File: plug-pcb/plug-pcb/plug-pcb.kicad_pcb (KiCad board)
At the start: 2 copper layers, 1 part, among them J2 Conn_01x05

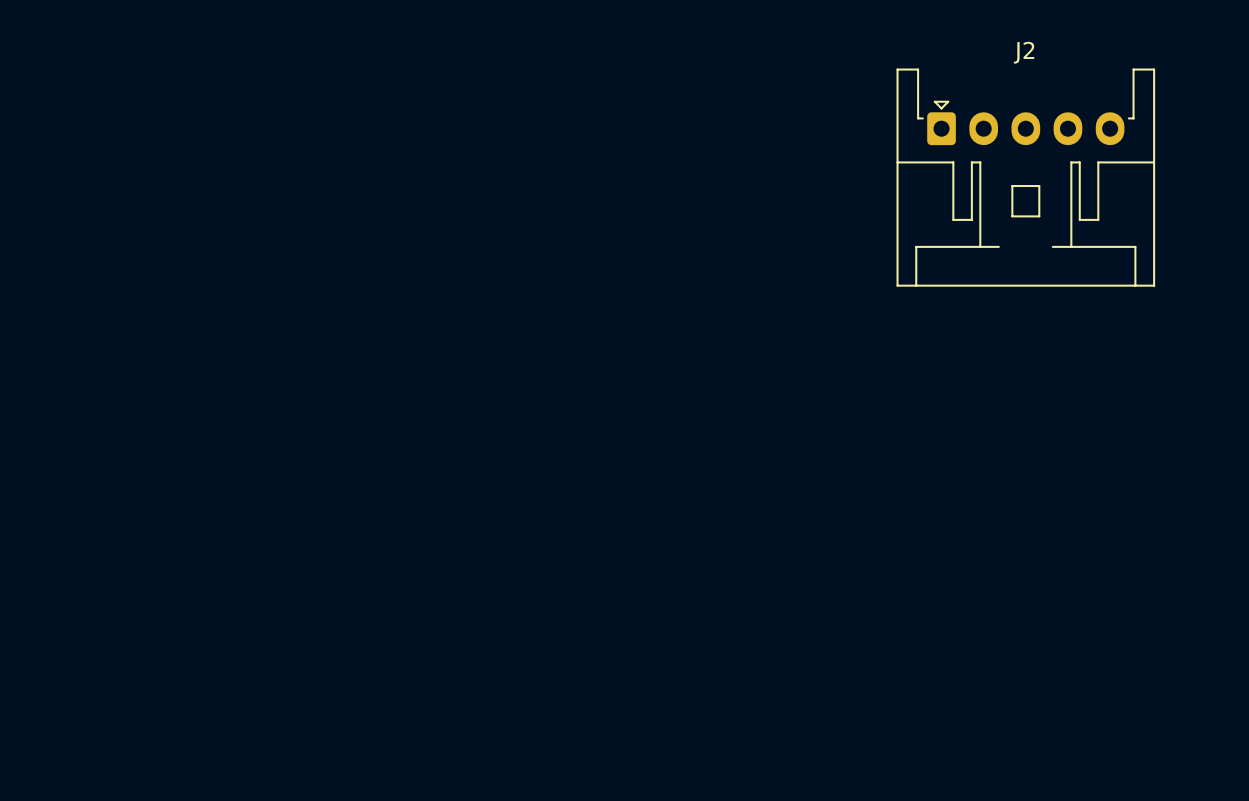
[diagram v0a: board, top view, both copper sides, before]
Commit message: WIP
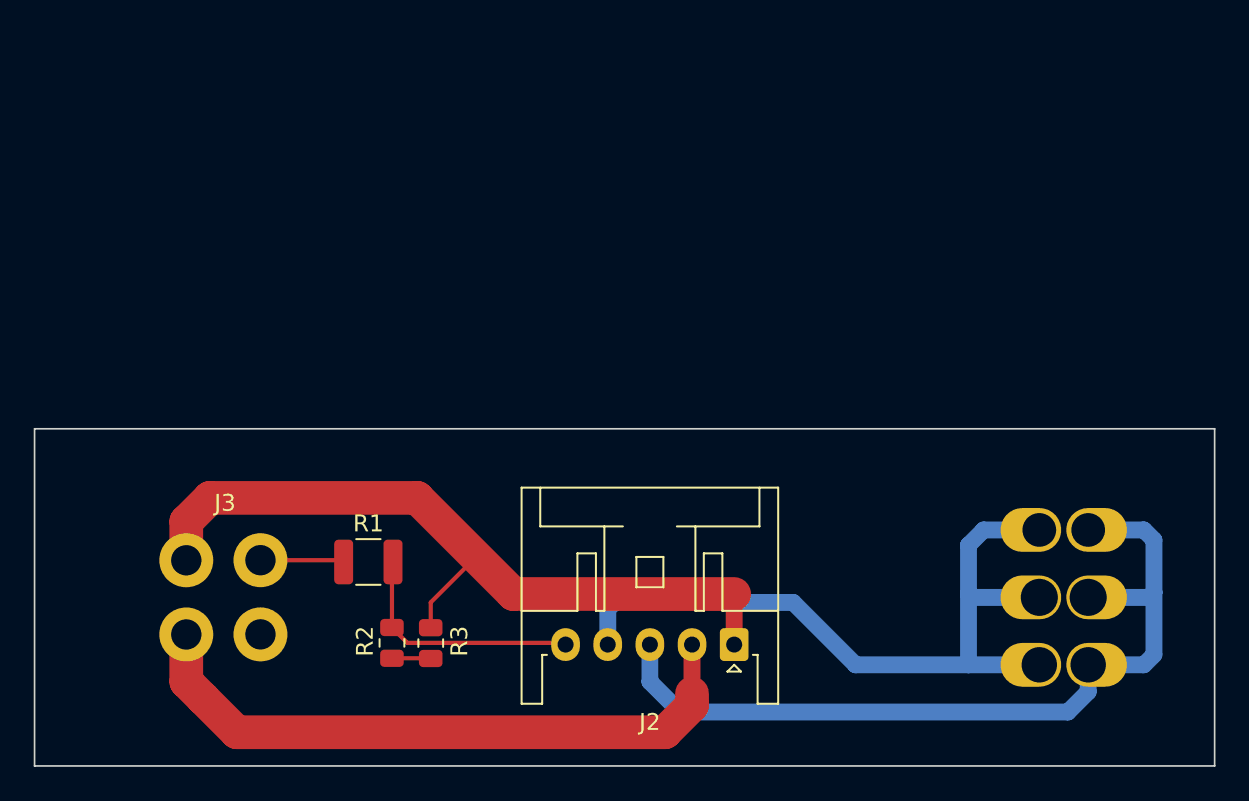
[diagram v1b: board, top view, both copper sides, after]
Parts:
- added J1: JCON_M12_02Pin, cacophony-footprints:jcon-2pin-m12, F.Cu at (142.5, 138.0)
- added J3: JCON_M16_04Pin, cacophony-footprints:jcon-4pin_m16, F.Cu at (89.0, 135.8)
- added R1: 2M, Resistor_SMD:R_1210_3225Metric, F.Cu at (99.8, 135.9)
- added R2: 150k, Resistor_SMD:R_0805_2012Metric, F.Cu at (101.2, 140.7)
- added R3: 22k, Resistor_SMD:R_0805_2012Metric, F.Cu at (103.5, 140.7)
- moved J2 33.0 mm to (121.5, 140.8), turned to 180 degrees
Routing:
- net /Speaker-: track 0.00 -> 50.2 mm
- net GND: track 0.00 -> 45.6 mm
- net /Speaker+: track 0.00 -> 45.4 mm
- net +12V: track 0.00 -> 38.3 mm
- net /Batt_sense: track 0.00 -> 14.6 mm
- net /+Batt: track 0.00 -> 4.98 mm
- net Net-(R2-Pad2): track 0.00 -> 2.31 mm
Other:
- board outline added: 70 x 20 mm

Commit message: WIP
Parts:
- removed J2: Conn_01x05, Connector_JST:JST_XA_S05B-XASK-1_1x05_P2.50mm_Horizontal
- added C101: 22uF, Capacitor_SMD:C_0805_2012Metric, F.Cu at (137.4, 124.5)
- added C102: 22uF, Capacitor_SMD:C_0805_2012Metric, F.Cu at (107.4, 127.0)
- added C103: 22uF, Capacitor_SMD:C_0805_2012Metric, F.Cu at (136.7, 127.3)
- added C104: 22uF, Capacitor_SMD:C_0805_2012Metric, F.Cu at (108.2, 124.0)
- added C105: 220uF, Capacitor_SMD:CP_Elec_8x10, F.Cu at (132.3, 146.5)
- added C106: 22uF, Capacitor_SMD:C_0805_2012Metric, F.Cu at (138.7, 127.3)
- added C107: 22uF, Capacitor_SMD:C_0805_2012Metric, F.Cu at (109.5, 127.0)
- added C108: 220uF, Capacitor_SMD:CP_Elec_8x10, F.Cu at (100.2, 146.3)
- added C109: 1nF, Capacitor_SMD:C_0402_1005Metric, F.Cu at (135.2, 127.0)
- added C110: 1nF, Capacitor_SMD:C_0402_1005Metric, F.Cu at (105.9, 126.8)
- added C111: 1nF, Capacitor_SMD:C_0402_1005Metric, F.Cu at (125.6, 129.1)
- added C112: 1nF, Capacitor_SMD:C_0402_1005Metric, F.Cu at (96.9, 125.6)
- added C113: 47pF, Capacitor_SMD:C_0402_1005Metric, F.Cu at (126.2, 126.6)
- added C114: 47pF, Capacitor_SMD:C_0402_1005Metric, F.Cu at (95.9, 127.7)
- added C115: 10nF, Capacitor_SMD:C_0402_1005Metric, F.Cu at (135.2, 124.0)
- added C116: 10nF, Capacitor_SMD:C_0402_1005Metric, F.Cu at (105.9, 124.0)
- added C117: 100nF, Capacitor_SMD:C_0402_1005Metric, F.Cu at (125.6, 131.5)
- added C118: 100nF, Capacitor_SMD:C_0402_1005Metric, F.Cu at (95.4, 130.2)
- added C119: 1nF, Capacitor_SMD:C_0402_1005Metric, F.Cu at (133.7, 130.6)
- added C120: 1nF, Capacitor_SMD:C_0402_1005Metric, F.Cu at (103.6, 130.5)
- added C121: 22uF, Capacitor_SMD:C_0603_1608Metric, F.Cu at (134.9, 130.6)
- added C122: 22uF, Capacitor_SMD:C_0603_1608Metric, F.Cu at (108.1, 130.5)
- added C123: 22uF, Capacitor_SMD:C_0603_1608Metric, F.Cu at (136.5, 130.6)
- added C124: 22uF, Capacitor_SMD:C_0603_1608Metric, F.Cu at (106.5, 130.5)
- added C125: 22uF, Capacitor_SMD:C_0603_1608Metric, F.Cu at (139.6, 130.6)
- added C126: 22uF, Capacitor_SMD:C_0603_1608Metric, F.Cu at (104.9, 130.5)
- added C127: 22uF, Capacitor_SMD:C_0603_1608Metric, F.Cu at (138.1, 130.6)
- added C128: 22uF, Capacitor_SMD:C_0603_1608Metric, F.Cu at (109.7, 130.5)
- added D101: D_Zener, cacophony-footprints:LL-34_L3.5-W1.5-RD, F.Cu at (108.1, 146.8)
- added D102: D_Shockley, Diode_SMD:D_SMA, F.Cu at (129.7, 130.3)
- added D103: D_Shockley, Diode_SMD:D_SMA, F.Cu at (99.5, 130.3)
- added J103: Conn_02x04_Odd_Even, cacophony-library:HDR-TH_8P-P2.54-H-F-R2-C4-S2.54-W10.2, F.Cu at (119.5, 148.6)
- added L101: 6.8uF, cacophony-footprints:IND-SMD_L8.0-W8.0_1217AS, F.Cu at (130.4, 137.3)
- added L102: 6.8uF, cacophony-footprints:IND-SMD_L8.0-W8.0_1217AS, F.Cu at (100.2, 136.9)
- added Q101: Q_PMOS_GSD, Package_TO_SOT_SMD:SOT-23, F.Cu at (108.6, 143.9)
- added R104: 100k, Resistor_SMD:R_0402_1005Metric, F.Cu at (106.1, 143.5)
- added R105: 33k, Resistor_SMD:R_0402_1005Metric, F.Cu at (126.2, 127.6)
- added R106: 33k, Resistor_SMD:R_0402_1005Metric, F.Cu at (96.9, 126.6)
- added R107: 150k, Resistor_SMD:R_0402_1005Metric, F.Cu at (126.2, 124.6)
- added R108: 22k, Resistor_SMD:R_0402_1005Metric, F.Cu at (96.9, 124.6)
- added R109: 10k, Resistor_SMD:R_0402_1005Metric, F.Cu at (95.4, 126.1)
- added R110: 100k, Resistor_SMD:R_0402_1005Metric, F.Cu at (126.2, 123.6)
- added R111: 22k, Resistor_SMD:R_0402_1005Metric, F.Cu at (126.2, 125.6)
- added R112: 100k, Resistor_SMD:R_0402_1005Metric, F.Cu at (96.9, 123.5)
- added U101: TPS54331, Package_SO:SO-8_3.9x4.9mm_P1.27mm, F.Cu at (130.9, 125.8)
- added U102: TPS54331, Package_SO:SO-8_3.9x4.9mm_P1.27mm, F.Cu at (101.7, 125.8)
- moved J102 22.8 mm to (111.4, 140.0), turned to 90 degrees
- moved R101 15.2 mm to (112.3, 144.5), turned to -90 degrees
- moved R102 13.3 mm to (112.4, 147.8), turned to 180 degrees
- moved R103 12.7 mm to (112.4, 149.8), turned to 0 degrees
- moved J101 5.48 mm to (137.2, 139.4), turned to 0 degrees
- renumbered J1 to J101, J3 to J102, R1 to R101, R2 to R102, R3 to R103
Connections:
- J102 pad 2: +12V -> VIN
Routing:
- net +3V3: track 0.00 -> 54.1 mm, vias 0 -> 7
- net +5V: track 0.00 -> 47.3 mm, vias 0 -> 2
- net 5V_EN: track 0.00 -> 36.0 mm, vias 0 -> 1
- net GND: track 45.6 -> 17.0 mm, vias 0 -> 32
- net +12V: track 38.3 -> 13.0 mm, vias 0 -> 23
- net /Speaker-: track 50.2 -> 26.5 mm
- net /Speaker+: track 45.4 -> 28.3 mm
- net Net-(C118-Pad1): track 0.00 -> 10.1 mm, vias 0 -> 2
- net Net-(C117-Pad1): track 0.00 -> 9.93 mm, vias 0 -> 2
- net VIN: track 0.00 -> 8.86 mm
- net /Batt_sense: track 14.6 -> 6.25 mm
- net Net-(D101-Pad2): track 0.00 -> 5.96 mm
- net /+Batt: track 4.98 -> 10.4 mm, vias 0 -> 1
- net Net-(R107-Pad2): track 0.00 -> 4.34 mm
- net Net-(C114-Pad1): track 0.00 -> 3.81 mm
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- added copper zone on F.Cu, net +12V
- added copper zone on In2.Cu, net +12V
- added copper zone on F.Cu, net +3V3
- added copper zone on F.Cu, net +5V
- added copper zone on F.Cu, net /SW_3V3
- added copper zone on F.Cu, net /SW_5V
- added copper zone on B.Cu, net GND
- added copper zone on F.Cu, net GND
- added copper zone on In1.Cu, net GND
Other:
- board size 70 x 20 mm -> 46.3 x 28.2 mm
- copper layers 2 -> 4
